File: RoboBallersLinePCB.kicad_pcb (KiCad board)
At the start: 2 copper layers, 132 x 132 mm, 117 parts, among them J1 Conn_01x04, J2 Bottom PCB, Q1 P-Channel, Q2 N-Channel, U1 MCP3008, U2 MCP3008, U3 MCP3008, U4 BoostConverter, U5 NSL-32, U6 NSL-32, U7 Solenoid-Electric

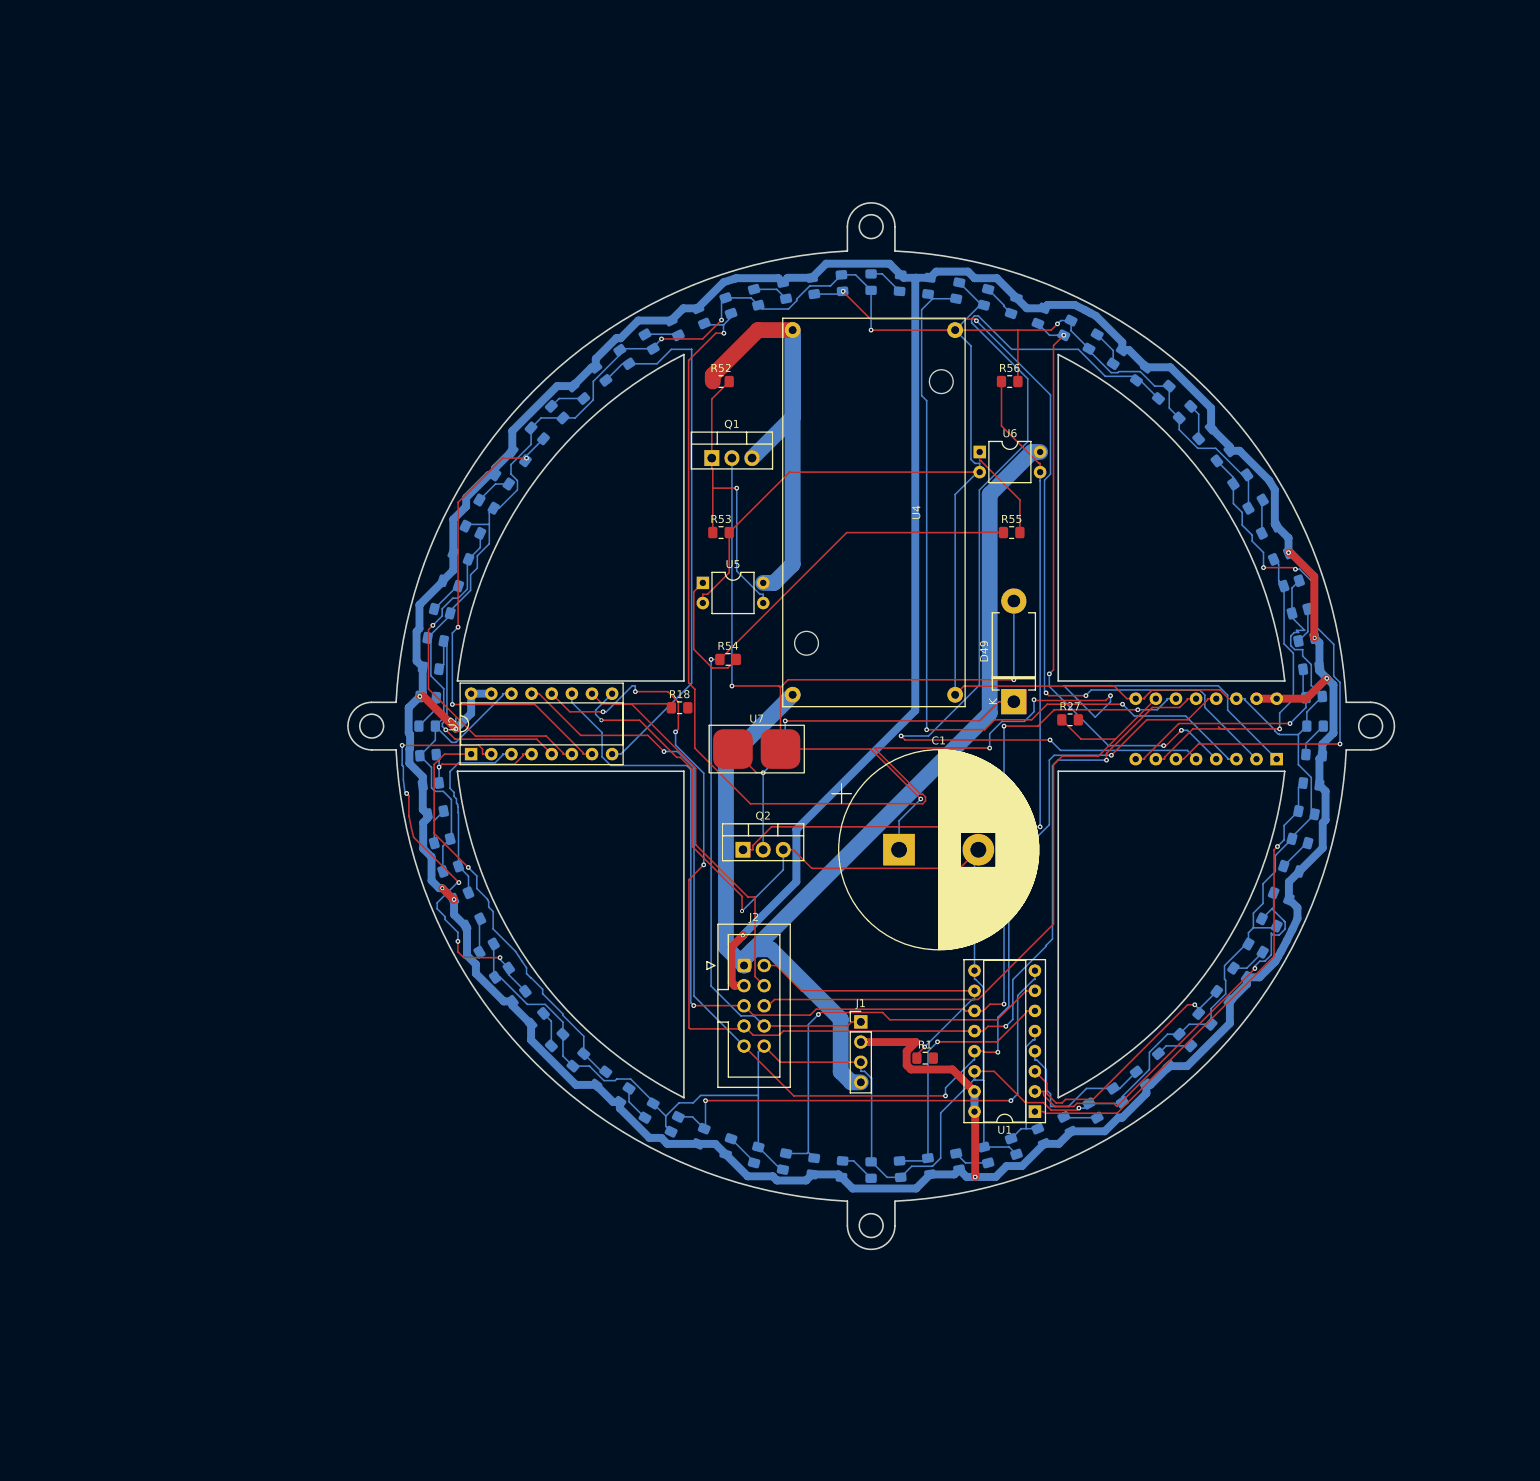
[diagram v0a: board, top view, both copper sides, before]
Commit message: spem needs to try
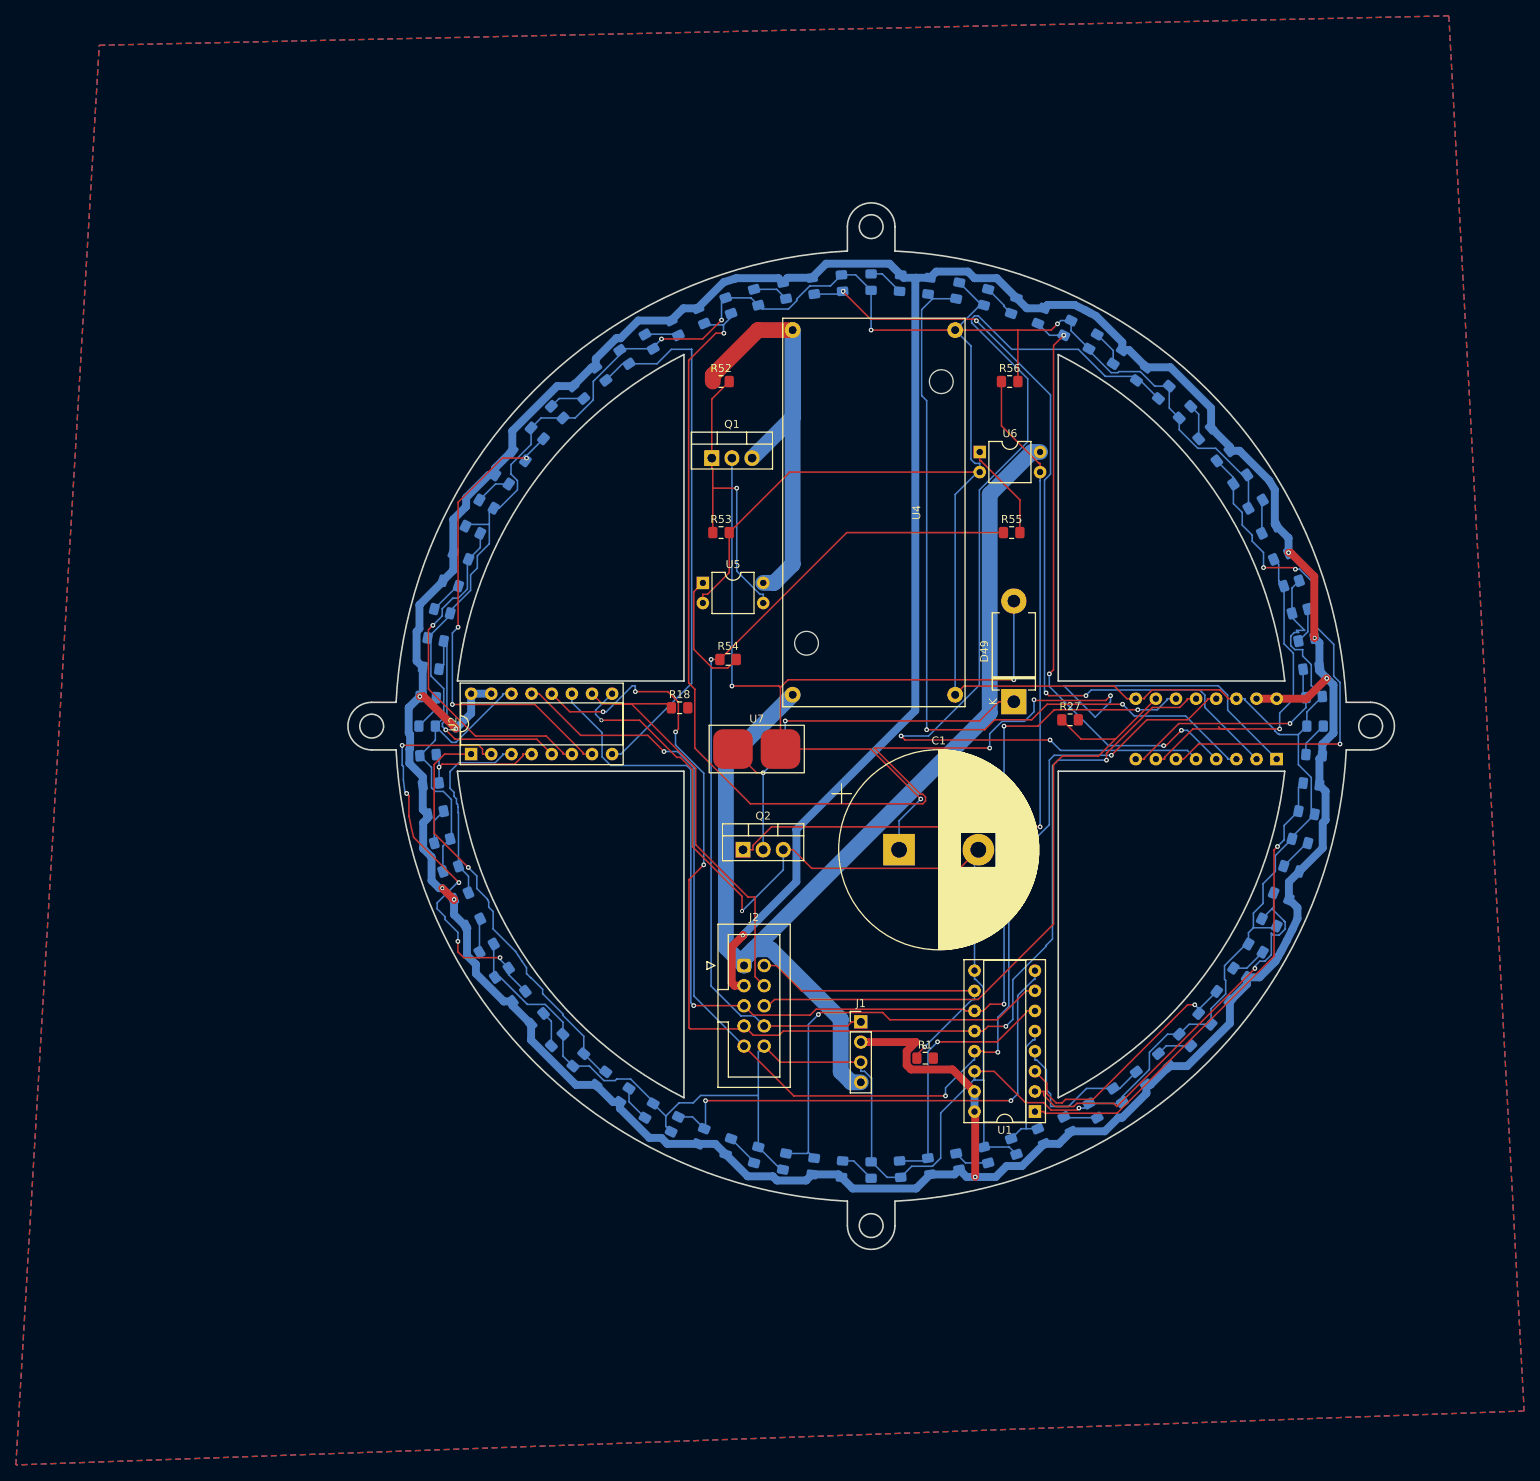
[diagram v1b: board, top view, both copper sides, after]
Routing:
- added copper zone on B.Cu, net GND
- added copper zone on F.Cu, net GND
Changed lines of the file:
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@@
 		(tags "Through hole vertical IDC box header THT 2x05 2.54mm double row")
 		(property "Reference" "J2"
-			(at 1.27 -6.1 360)
+			(at 1.27 -6.1 0)
 			(layer "F.SilkS")
 			(effects
@@
 		)
 		(property "Value" "Bottom PCB"
-			(at 1.27 16.26 360)
+			(at 1.27 16.26 0)
 			(layer "F.Fab")
 			(effects
@@
 		(net 68)
 	)
+	(zone
+		(net 2)
+		(net_name "GND")
+		(layers "F&B.Cu")
+		(hatch edge 0.5)
+		(connect_pads
+			(clearance 0.5)
+		)
+		(min_thickness 0.25)
+		(filled_areas_thickness no)
+		(fill yes
+			(thermal_gap 0.5)
+			(thermal_bridge_width 0.5)
+		)
+		(polygon
+			(pts
+				(xy 202.6412 214.122) (xy 372.872 210.4136) (xy 382.3716 386.3848) (xy 192.1256 393.192)
+			)
+		)
+	)
 	(group ""
